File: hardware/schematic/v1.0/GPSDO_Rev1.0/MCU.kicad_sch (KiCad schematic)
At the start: 7 parts, among them U1 TDC7200PWR, U9 STM32G431KBUx

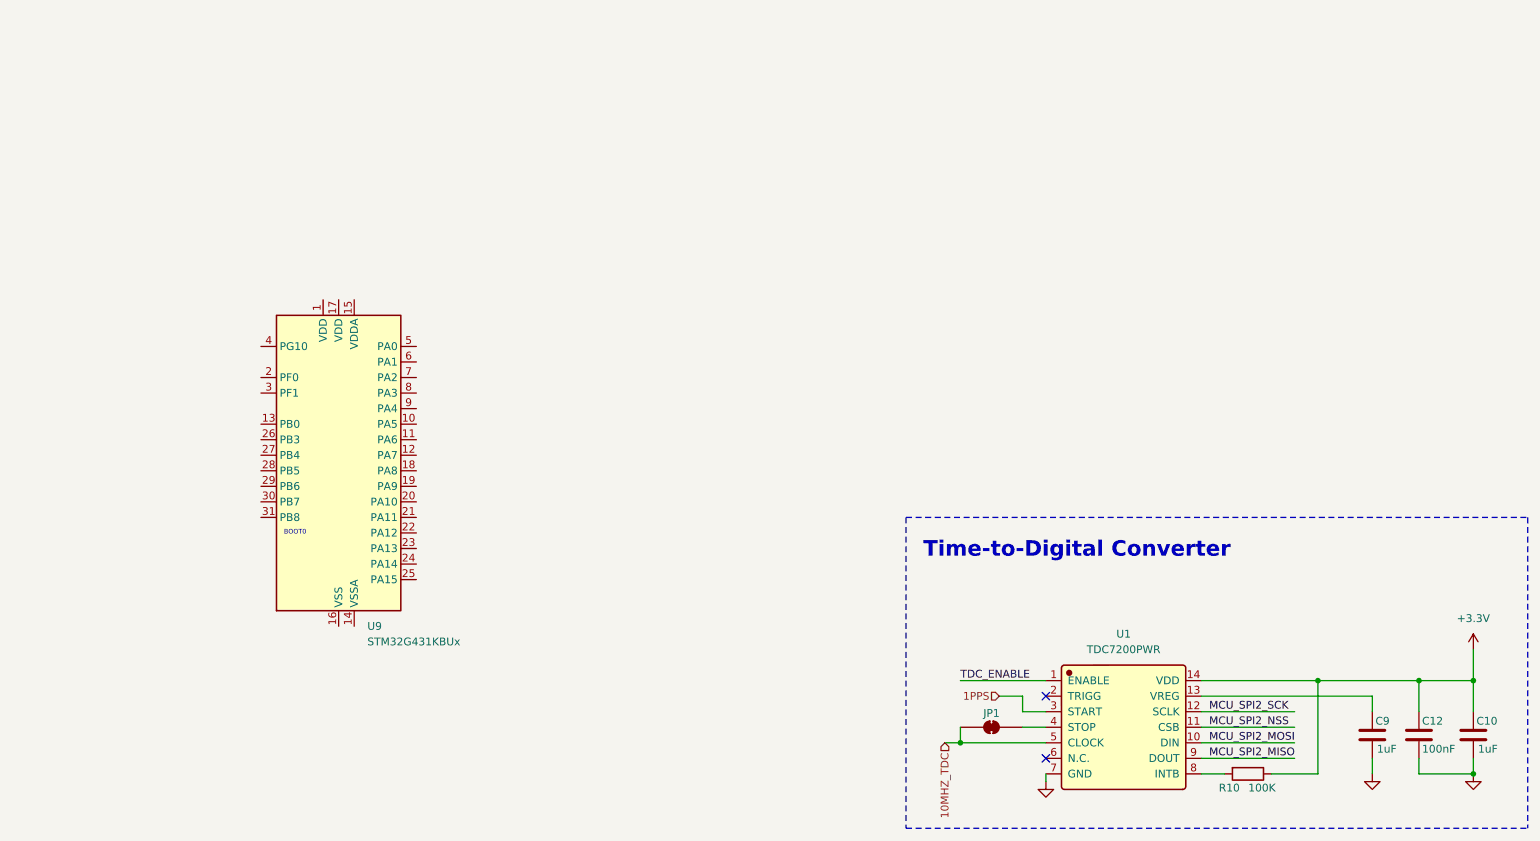
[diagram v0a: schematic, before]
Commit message: pdf and sch update
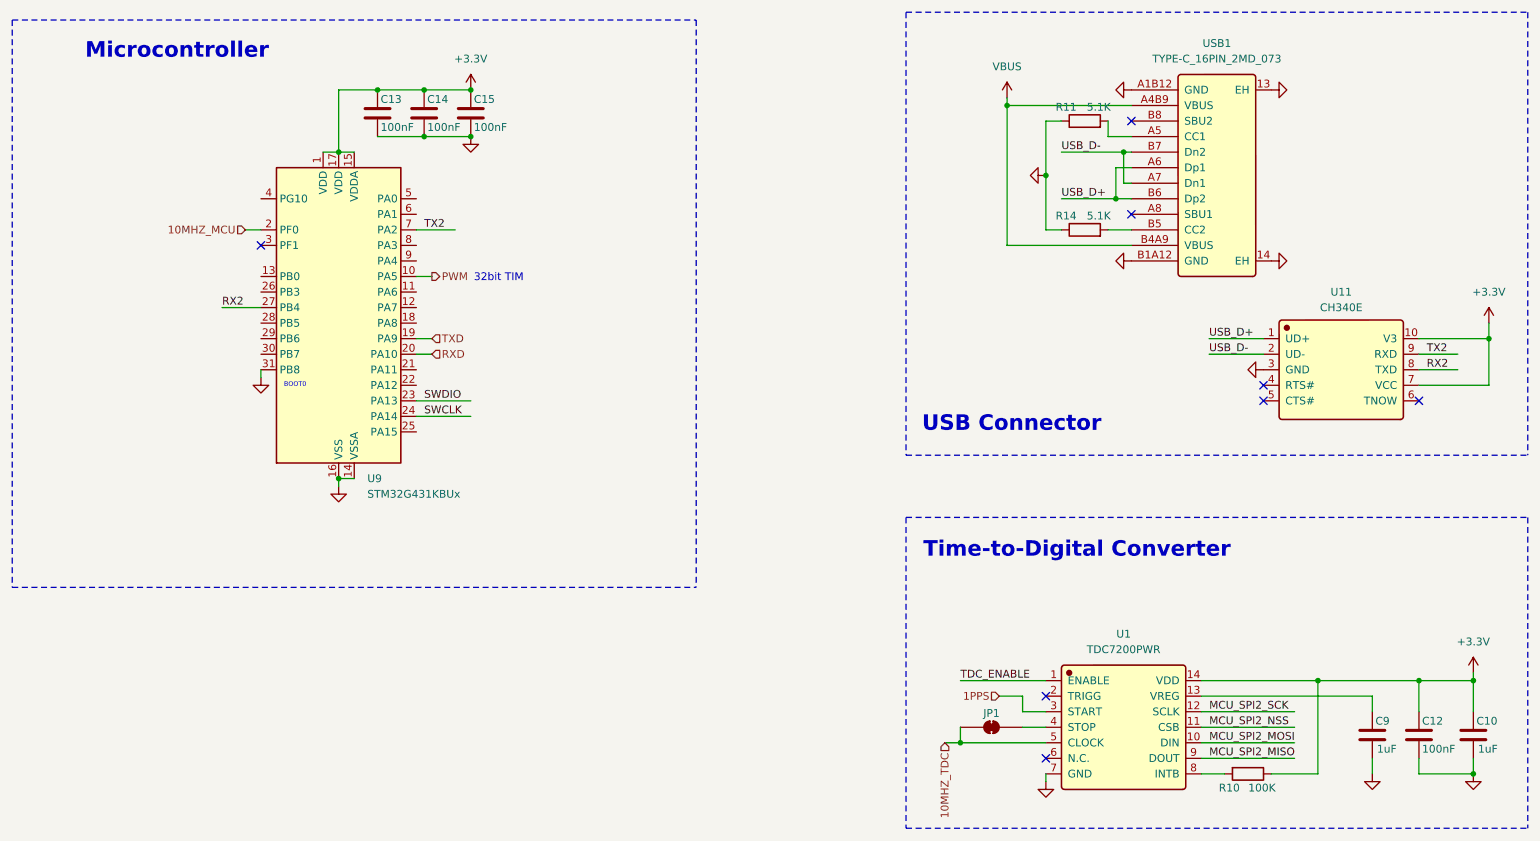
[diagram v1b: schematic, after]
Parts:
- added C13, C14, C15: 100nF, GPSDO_Rev1.0:C_0402_1005Metric, symbol GPSDO_Rev1.0:C
- added R11, R14: 5.1K, GPSDO_Rev1.0:R_0402_1005Metric, symbol GPSDO_Rev1.0:R
- added U11: CH340E, GPSDO_Rev1.0:CH340E, symbol GPSDO_Rev1.0:CH340E
- added USB1: TYPE-C_16PIN_2MD_073, GPSDO_Rev1.0:TYPE-C_16PIN_2MD_073, symbol GPSDO_Rev1.0:TYPE-C_16PIN_2MD_073
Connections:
- net +3.3V: now also U9.1 (VDD), U9.15 (VDDA), U9.17 (VDD), C13.1, C14.1, C15.1, U11.10 (V3), U11.7 (VCC)
- net GND: now also U9.14 (VSSA), U9.16 (VSS), U9.31 (PB8), U9.32 (VSS), U9.33 (VSS), C13.2, C14.2, C15.2, R11.1, R14.1, U11.3 (GND), USB1.13 (EH), USB1.14 (EH), USB1.A1B12 (GND), USB1.B1A12 (GND)
- net PWM: now reaches U9.10 (PA5)
- net TXD: now reaches U9.19 (PA9)
- net 10MHZ_MCU: now reaches U9.2 (PF0)
- net RXD: now reaches U9.20 (PA10)
- net SWDIO: now reaches U9.23 (PA13)
- net SWCLK: now reaches U9.24 (PA14)
- net RX2: now reaches U9.27 (PB4)
- net RX2: now also U11.8 (TXD)
- net TX2: now reaches U9.7 (PA2)
- net TX2: now also U11.9 (RXD)
- new net: R11.2, USB1.A5 (CC1)
- new net: R14.2, USB1.B5 (CC2)
- new net USB_D+: U11.1 (UD+), USB1.A6 (Dp1), USB1.B6 (Dp2)
- new net USB_D-: U11.2 (UD-), USB1.A7 (Dn1), USB1.B7 (Dn2)
- new net VBUS: USB1.A4B9 (VBUS), USB1.B4A9 (VBUS)
- no-connect marks 2 -> 8
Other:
- note added: "32bit TIM"
- note added: "Microcontroller"
- note added: "USB Connector"
- moved on the sheet: U9
